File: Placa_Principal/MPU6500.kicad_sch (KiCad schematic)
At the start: 1 part, among them U6 GY-6500 MPU6500

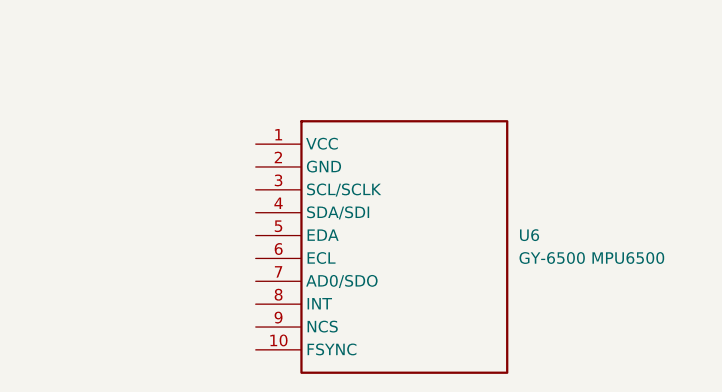
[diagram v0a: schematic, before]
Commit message: Segundo commit
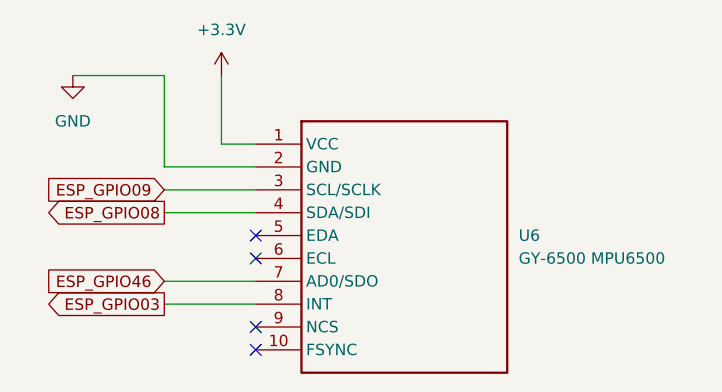
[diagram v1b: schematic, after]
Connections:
- net +3.3V: now reaches U6.1 (VCC)
- net GND: now reaches U6.2 (GND)
- net ESP_GPIO09: now reaches U6.3 (SCL/SCLK)
- net ESP_GPIO08: now reaches U6.4 (SDA/SDI)
- net ESP_GPIO46: now reaches U6.7 (AD0/SDO)
- net ESP_GPIO03: now reaches U6.8 (INT)
- no-connect marks 0 -> 4
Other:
- company: (none) -> Titans Robotic Team
- title: (none) -> Conexões MPU6500 - SSL-EL  2026
